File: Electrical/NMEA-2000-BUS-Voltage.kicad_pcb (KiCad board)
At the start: 2 copper layers, 52.1 x 40.6 mm, 12 parts, among them J1 Conn_01x06, SW1 SW_Push, U1 WeMos_D1_mini, U2 LM7805_TO220

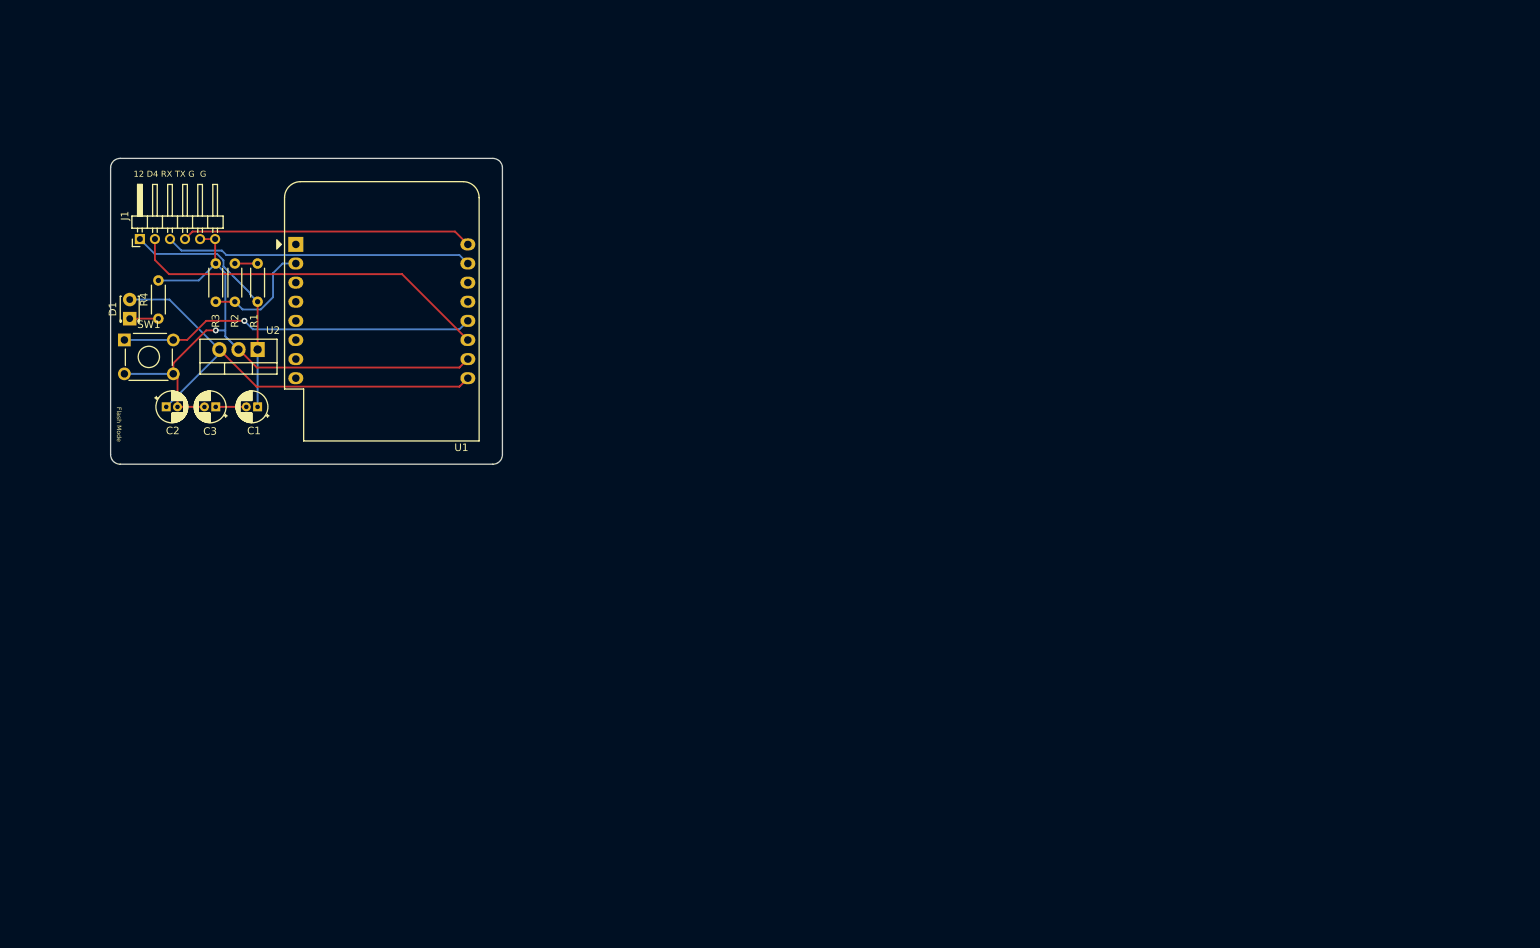
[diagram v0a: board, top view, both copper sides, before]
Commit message: Updated PCB
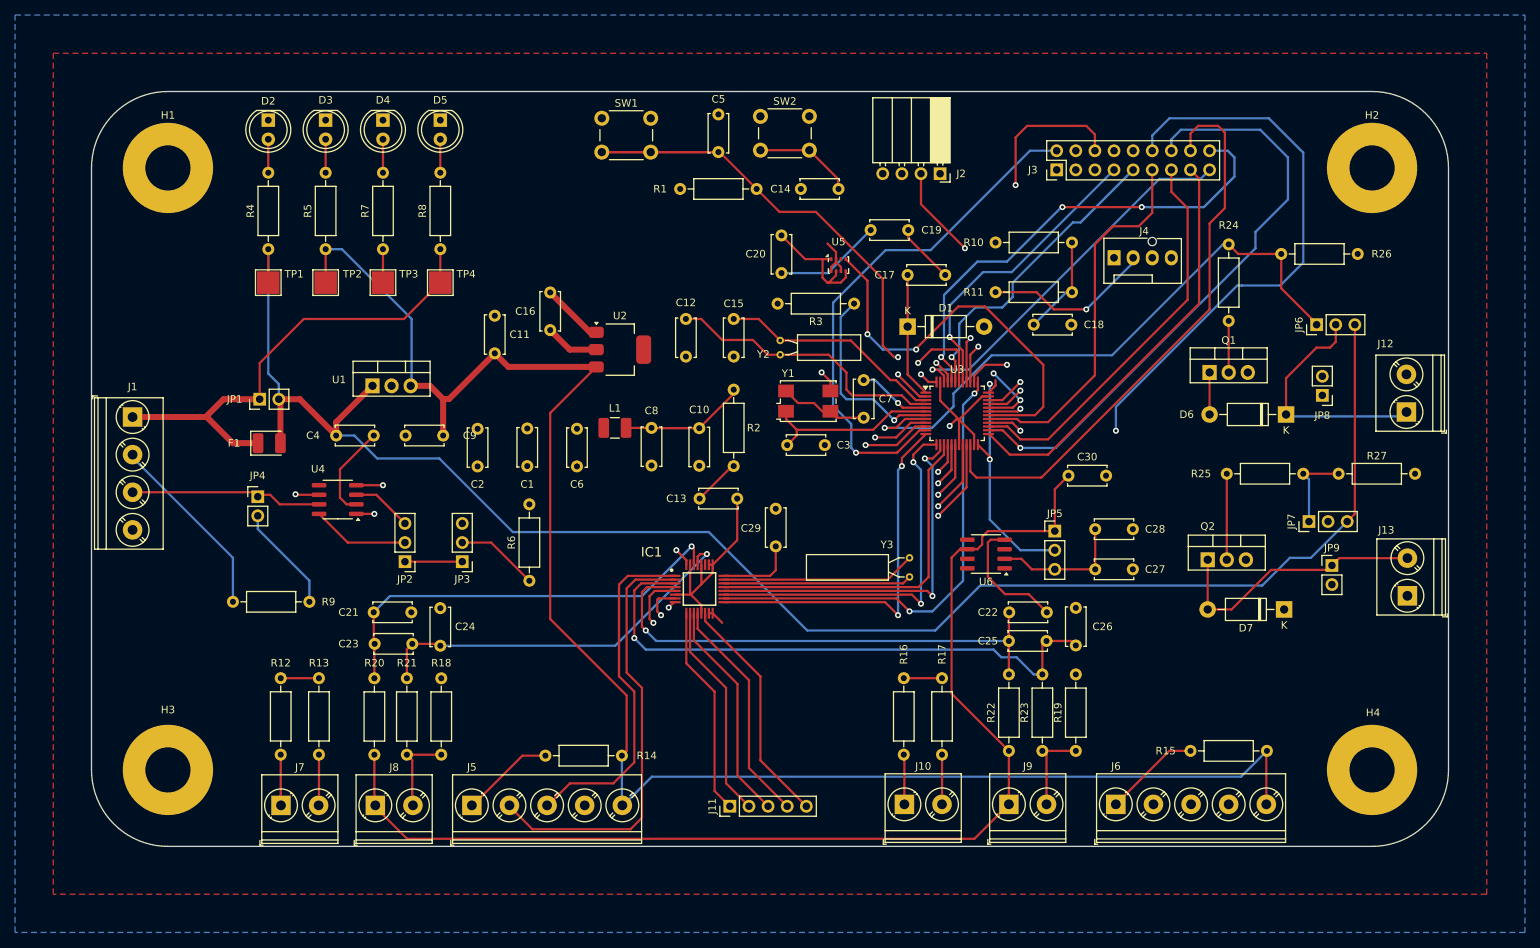
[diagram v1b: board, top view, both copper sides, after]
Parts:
- added C10: 1uF, Capacitor_THT:C_Disc_D5.0mm_W2.5mm_P5.00mm, F.Cu at (139.2, 85.4)
- added C11: 0.33uF, Capacitor_THT:C_Disc_D5.0mm_W2.5mm_P5.00mm, F.Cu at (112.0, 75.4)
- added C12: 20pF, Capacitor_THT:C_Disc_D5.0mm_W2.5mm_P5.00mm, F.Cu at (137.4, 70.9)
- added C13: 0.1uF, Capacitor_THT:C_Disc_D5.0mm_W2.5mm_P5.00mm, F.Cu at (139.2, 94.7)
- added C14: 0.1uF, Capacitor_THT:C_Disc_D5.0mm_W2.5mm_P5.00mm, F.Cu at (152.7, 53.6)
- added C15: 20pF, Capacitor_THT:C_Disc_D5.0mm_W2.5mm_P5.00mm, F.Cu at (143.8, 70.9)
- added C16: 0.1uF, Capacitor_THT:C_Disc_D5.0mm_W2.5mm_P5.00mm, F.Cu at (119.4, 72.3)
- added C17: 0.1uF, Capacitor_THT:C_Disc_D5.0mm_W2.5mm_P5.00mm, F.Cu at (166.9, 65.0)
- added C18: 0.1nF, Capacitor_THT:C_Disc_D5.0mm_W2.5mm_P5.00mm, F.Cu at (183.6, 71.6)
- added C19: 0.1uF, Capacitor_THT:C_Disc_D5.0mm_W2.5mm_P5.00mm, F.Cu at (162.0, 59.1)
- added C20: 0.1uF, Capacitor_THT:C_Disc_D5.0mm_W2.5mm_P5.00mm, F.Cu at (150.1, 64.8)
- added C21: 10nF, Capacitor_THT:C_Disc_D5.0mm_W2.5mm_P5.00mm, F.Cu at (95.9, 109.9)
- added C22: 10nF, Capacitor_THT:C_Disc_D5.0mm_W2.5mm_P5.00mm, F.Cu at (180.4, 109.9)
- added C23: 0.1uF, Capacitor_THT:C_Disc_D5.0mm_W2.5mm_P5.00mm, F.Cu at (96.1, 114.0)
- added C24: 10nF, Capacitor_THT:C_Disc_D5.0mm_W2.5mm_P5.00mm, F.Cu at (104.8, 114.3)
- added C25: 0.1uF, Capacitor_THT:C_Disc_D5.0mm_W2.5mm_P5.00mm, F.Cu at (180.3, 113.7)
- added C26: 10nF, Capacitor_THT:C_Disc_D5.0mm_W2.5mm_P5.00mm, F.Cu at (189.2, 114.3)
- added C27: 1uF, Capacitor_THT:C_Disc_D5.0mm_W2.5mm_P5.00mm, F.Cu at (191.8, 104.1)
- added C28: 0.1uF, Capacitor_THT:C_Disc_D5.0mm_W2.5mm_P5.00mm, F.Cu at (191.8, 98.8)
- added C29: 220nF, Capacitor_THT:C_Disc_D5.0mm_W2.5mm_P5.00mm, F.Cu at (149.4, 101.1)
- added C30: 0.1uF, Capacitor_THT:C_Disc_D5.0mm_W2.5mm_P5.00mm, F.Cu at (188.3, 91.7)
- added C4: 0.33uF, Capacitor_THT:C_Disc_D5.0mm_W2.5mm_P5.00mm, F.Cu at (90.9, 86.4)
- added C5: 0.1uF, Capacitor_THT:C_Disc_D5.0mm_W2.5mm_P5.00mm, F.Cu at (141.7, 43.7)
- added C6: 0.1uF, Capacitor_THT:C_Disc_D5.0mm_W2.5mm_P5.00mm, F.Cu at (122.9, 85.5)
- added C7: 20pF, Capacitor_THT:C_Disc_D5.0mm_W2.5mm_P5.00mm, F.Cu at (161.0, 79.0)
- added C8: 10nF, Capacitor_THT:C_Disc_D5.0mm_W2.5mm_P5.00mm, F.Cu at (132.8, 85.3)
- added C9: 0.1uF, Capacitor_THT:C_Disc_D5.0mm_W2.5mm_P5.00mm, F.Cu at (105.2, 86.4)
- added D2: LED, LED_THT:LED_D5.0mm, F.Cu at (81.9, 44.5)
- added D3: LED, LED_THT:LED_D5.0mm, F.Cu at (89.5, 44.4)
- added D4: LED, LED_THT:LED_D5.0mm, F.Cu at (97.2, 44.5)
- added D5: LED, LED_THT:LED_D5.0mm, F.Cu at (104.8, 44.5)
- added D6: 1N5819, Diode_THT:D_DO-41_SOD81_P10.16mm_Horizontal, F.Cu at (217.2, 83.6)
- added D7: 1N5819, Diode_THT:D_DO-41_SOD81_P10.16mm_Horizontal, F.Cu at (216.9, 109.5)
- added F1: Polyfuse, Diode_SMD:D_1210_3225Metric_Pad1.42x2.65mm_HandSolder, F.Cu at (82.0, 87.4)
- added H1: MountingHole_Pad, MountingHole:MountingHole_6mm_Pad, F.Cu at (68.6, 50.8)
- added H2: MountingHole_Pad, MountingHole:MountingHole_6mm_Pad, F.Cu at (228.6, 50.8)
- added H3: MountingHole_Pad, MountingHole:MountingHole_6mm_Pad, F.Cu at (68.6, 130.8)
- added H4: MountingHole_Pad, MountingHole:MountingHole_6mm_Pad, F.Cu at (228.6, 130.8)
- added IC1: ADS131M08, ADS131M08QPBSRQ1:QFP50P700X700X120-32N, F.Cu at (139.2, 106.8)
- added J10: Conn_01x02, TerminalBlock_Phoenix:TerminalBlock_Phoenix_PT-1,5-2-5.0-H_1x02_P5.00mm_Horizontal, F.Cu at (166.4, 135.4)
- added J11: Conn_01x05, Connector_PinHeader_2.54mm:PinHeader_1x05_P2.54mm_Vertical, F.Cu at (143.3, 135.6)
- added J12: Conn_01x02, TerminalBlock_Phoenix:TerminalBlock_Phoenix_PT-1,5-2-5.0-H_1x02_P5.00mm_Horizontal, F.Cu at (233.2, 83.2)
- added J13: Conn_01x02, TerminalBlock_Phoenix:TerminalBlock_Phoenix_PT-1,5-2-5.0-H_1x02_P5.00mm_Horizontal, F.Cu at (233.3, 107.7)
- added J2: Conn_01x04, Connector_PinSocket_2.54mm:PinSocket_1x04_P2.54mm_Horizontal, F.Cu at (171.2, 51.6)
- added J3: Conn_02x08_Counter_Clockwise, Connector_PinHeader_2.54mm:PinHeader_2x09_P2.54mm_Vertical, F.Cu at (186.7, 51.1)
- added J4: Conn_01x04, Connector:FanPinHeader_1x04_P2.54mm_Vertical, F.Cu at (194.3, 62.7)
- added J5: Conn_01x05, TerminalBlock_Phoenix:TerminalBlock_Phoenix_PT-1,5-5-5.0-H_1x05_P5.00mm_Horizontal, F.Cu at (109.0, 135.5)
- added J6: Conn_01x05, TerminalBlock_Phoenix:TerminalBlock_Phoenix_PT-1,5-5-5.0-H_1x05_P5.00mm_Horizontal, F.Cu at (194.6, 135.4)
- added J7: Conn_01x02, TerminalBlock_Phoenix:TerminalBlock_Phoenix_PT-1,5-2-5.0-H_1x02_P5.00mm_Horizontal, F.Cu at (83.6, 135.5)
- added J8: Conn_01x02, TerminalBlock_Phoenix:TerminalBlock_Phoenix_PT-1,5-2-5.0-H_1x02_P5.00mm_Horizontal, F.Cu at (96.1, 135.5)
- added J9: Conn_01x02, TerminalBlock_Phoenix:TerminalBlock_Phoenix_PT-1,5-2-5.0-H_1x02_P5.00mm_Horizontal, F.Cu at (180.3, 135.4)
- added JP1: Jumper_2_Open, Connector_PinHeader_2.54mm:PinHeader_1x02_P2.54mm_Vertical, F.Cu at (80.8, 81.5)
- added JP2: Jumper_3_Bridged12, Connector_PinHeader_2.54mm:PinHeader_1x03_P2.54mm_Vertical, F.Cu at (100.1, 103.1)
- added JP3: Jumper_3_Bridged12, Connector_PinHeader_2.54mm:PinHeader_1x03_P2.54mm_Vertical, F.Cu at (107.7, 103.1)
- added JP4: Jumper_2_Open, Connector_PinHeader_2.54mm:PinHeader_1x02_P2.54mm_Vertical, F.Cu at (80.5, 94.5)
- added JP5: Jumper_3_Bridged12, Connector_PinHeader_2.54mm:PinHeader_1x03_P2.54mm_Vertical, F.Cu at (186.4, 99.1)
- added JP6: Jumper_3_Bridged12, Connector_PinHeader_2.54mm:PinHeader_1x03_P2.54mm_Vertical, F.Cu at (221.2, 71.6)
- added JP7: Jumper_3_Bridged12, Connector_PinHeader_2.54mm:PinHeader_1x03_P2.54mm_Vertical, F.Cu at (220.2, 97.8)
- added JP8: Jumper_2_Bridged, Connector_PinHeader_2.54mm:PinHeader_1x02_P2.54mm_Vertical, F.Cu at (222.0, 81.0)
- added JP9: Jumper_2_Bridged, Connector_PinHeader_2.54mm:PinHeader_1x02_P2.54mm_Vertical, F.Cu at (223.3, 103.6)
- added L1: CBG322513U102T, Inductor_SMD:L_1210_3225Metric_Pad1.42x2.65mm_HandSolder, F.Cu at (128.0, 85.3)
- added Q1: IRFZ44N, Package_TO_SOT_THT:TO-220-3_Vertical, F.Cu at (207.0, 78.0)
- added Q2: IRFZ44N, Package_TO_SOT_THT:TO-220-3_Vertical, F.Cu at (206.8, 102.9)
- added R10: 10k, Resistor_THT:R_Axial_DIN0207_L6.3mm_D2.5mm_P10.16mm_Horizontal, F.Cu at (178.6, 60.7)
- added R11: 3.3k, Resistor_THT:R_Axial_DIN0207_L6.3mm_D2.5mm_P10.16mm_Horizontal, F.Cu at (188.7, 67.3)
- added R12: 10k, Resistor_THT:R_Axial_DIN0207_L6.3mm_D2.5mm_P10.16mm_Horizontal, F.Cu at (83.6, 128.8)
- added R13: 4k7, Resistor_THT:R_Axial_DIN0207_L6.3mm_D2.5mm_P10.16mm_Horizontal, F.Cu at (88.6, 118.6)
- added R14: 10k, Resistor_THT:R_Axial_DIN0207_L6.3mm_D2.5mm_P10.16mm_Horizontal, F.Cu at (128.9, 128.9)
- added R15: 10k, Resistor_THT:R_Axial_DIN0207_L6.3mm_D2.5mm_P10.16mm_Horizontal, F.Cu at (204.5, 128.3)
- added R16: 10k, Resistor_THT:R_Axial_DIN0207_L6.3mm_D2.5mm_P10.16mm_Horizontal, F.Cu at (166.4, 128.8)
- added R17: 4k7, Resistor_THT:R_Axial_DIN0207_L6.3mm_D2.5mm_P10.16mm_Horizontal, F.Cu at (171.4, 118.6)
- added R18: 10k, Resistor_THT:R_Axial_DIN0207_L6.3mm_D2.5mm_P10.16mm_Horizontal, F.Cu at (104.9, 128.8)
- added R19: 10k, Resistor_THT:R_Axial_DIN0207_L6.3mm_D2.5mm_P10.16mm_Horizontal, F.Cu at (189.2, 128.3)
- added R20: 1k, Resistor_THT:R_Axial_DIN0207_L6.3mm_D2.5mm_P10.16mm_Horizontal, F.Cu at (96.0, 128.8)
- added R21: 1k, Resistor_THT:R_Axial_DIN0207_L6.3mm_D2.5mm_P10.16mm_Horizontal, F.Cu at (100.3, 128.8)
- added R22: 1k, Resistor_THT:R_Axial_DIN0207_L6.3mm_D2.5mm_P10.16mm_Horizontal, F.Cu at (180.3, 128.3)
- added R23: 1k, Resistor_THT:R_Axial_DIN0207_L6.3mm_D2.5mm_P10.16mm_Horizontal, F.Cu at (184.8, 128.3)
- added R24: 120R, Resistor_THT:R_Axial_DIN0207_L6.3mm_D2.5mm_P10.16mm_Horizontal, F.Cu at (209.6, 61.0)
- added R25: 120R, Resistor_THT:R_Axial_DIN0207_L6.3mm_D2.5mm_P10.16mm_Horizontal, F.Cu at (219.5, 91.4)
- added R26: 10k, Resistor_THT:R_Axial_DIN0207_L6.3mm_D2.5mm_P10.16mm_Horizontal, F.Cu at (216.5, 62.2)
- added R27: 10k, Resistor_THT:R_Axial_DIN0207_L6.3mm_D2.5mm_P10.16mm_Horizontal, F.Cu at (224.2, 91.4)
- added R5: 470R, Resistor_THT:R_Axial_DIN0207_L6.3mm_D2.5mm_P10.16mm_Horizontal, F.Cu at (89.5, 61.6)
- added R6: 10k, Resistor_THT:R_Axial_DIN0207_L6.3mm_D2.5mm_P10.16mm_Horizontal, F.Cu at (116.6, 105.7)
- added R7: 330R, Resistor_THT:R_Axial_DIN0207_L6.3mm_D2.5mm_P10.16mm_Horizontal, F.Cu at (97.2, 61.6)
- added R8: 1k5, Resistor_THT:R_Axial_DIN0207_L6.3mm_D2.5mm_P10.16mm_Horizontal, F.Cu at (104.8, 61.6)
- added R9: 120R, Resistor_THT:R_Axial_DIN0207_L6.3mm_D2.5mm_P10.16mm_Horizontal, F.Cu at (87.4, 108.5)
- added SW2: SW_Push, Button_Switch_THT:SW_PUSH_6mm, F.Cu at (147.3, 43.9)
- added TP1: 12V, TestPoint:TestPoint_Pad_3.0x3.0mm, F.Cu at (81.9, 66.0)
- added TP2: 5V, TestPoint:TestPoint_Pad_3.0x3.0mm, F.Cu at (89.5, 66.0)
- added TP3: 3.3V, TestPoint:TestPoint_Pad_3.0x3.0mm, F.Cu at (97.2, 66.0)
- added TP4: VMot, TestPoint:TestPoint_Pad_3.0x3.0mm, F.Cu at (104.8, 66.0)
- added U3: STM32G431CBTx, Package_QFP:LQFP-48_7x7mm_P0.5mm, F.Cu at (173.5, 83.4)
- added U4: SN65HVD230, Package_SO:SOIC-8_3.9x4.9mm_P1.27mm, F.Cu at (91.1, 94.9)
- added U5: BMP280, N2K-influx:Bosch_LGA-8_2x2.5mm_P0.65mm_ClockwisePinNumbering, F.Cu at (157.7, 63.7)
- added U6: ADR4533, Package_SO:SOIC-8_3.9x4.9mm_P1.27mm, F.Cu at (177.3, 102.1)
- added Y1: K7A080002020, Crystal:Crystal_SMD_7050-4Pin_7.0x5.0mm, F.Cu at (153.7, 81.8)
- added Y2: X308032768KGB2SC, Crystal:Crystal_C38-LF_D3.0mm_L8.0mm_Horizontal, F.Cu at (149.9, 75.6)
- added Y3: 20kHz Crystal, Crystal:Crystal_AT310_D3.0mm_L10.0mm_Horizontal, F.Cu at (167.1, 102.6)
- C1: value 0.2uF -> 0.1uF; footprint Capacitor_THT:CP_Radial_D4.0mm_P1.50mm -> Capacitor_THT:C_Disc_D5.0mm_W2.5mm_P5.00mm
- C2: footprint Capacitor_THT:CP_Radial_D4.0mm_P1.50mm -> Capacitor_THT:C_Disc_D5.0mm_W2.5mm_P5.00mm
- C3: value 0.1uF -> 20pF; footprint Capacitor_THT:CP_Radial_D4.0mm_P1.50mm -> Capacitor_THT:C_Disc_D5.0mm_W2.5mm_P5.00mm
- D1: value LED -> 1N5819; footprint LED_THT:LED_D1.8mm_W3.3mm_H2.4mm -> Diode_THT:D_DO-41_SOD81_P10.16mm_Horizontal
- J1: value Conn_01x06 -> Conn_01x04; footprint Connector_PinHeader_2.00mm:PinHeader_1x06_P2.00mm_Horizontal -> TerminalBlock_Phoenix:TerminalBlock_Phoenix_PT-1,5-4-5.0-H_1x04_P5.00mm_Horizontal
- R1: footprint Resistor_THT:R_Axial_DIN0204_L3.6mm_D1.6mm_P5.08mm_Horizontal -> Resistor_THT:R_Axial_DIN0207_L6.3mm_D2.5mm_P10.16mm_Horizontal
- R2: value 20k -> 0R; footprint Resistor_THT:R_Axial_DIN0204_L3.6mm_D1.6mm_P5.08mm_Horizontal -> Resistor_THT:R_Axial_DIN0207_L6.3mm_D2.5mm_P10.16mm_Horizontal
- R3: value 120k -> 10k; footprint Resistor_THT:R_Axial_DIN0204_L3.6mm_D1.6mm_P5.08mm_Horizontal -> Resistor_THT:R_Axial_DIN0207_L6.3mm_D2.5mm_P10.16mm_Horizontal
- R4: value 1k -> 1.2k; footprint Resistor_THT:R_Axial_DIN0204_L3.6mm_D1.6mm_P5.08mm_Horizontal -> Resistor_THT:R_Axial_DIN0207_L6.3mm_D2.5mm_P10.16mm_Horizontal
- SW1: footprint Button_Switch_THT:SW_TH_Tactile_Omron_B3F-10xx -> Button_Switch_THT:SW_PUSH_6mm
- U1: value WeMos_D1_mini -> LM7805_TO220; footprint Module:WEMOS_D1_mini_light -> Package_TO_SOT_THT:TO-220-3_Vertical
- U2: value LM7805_TO220 -> AMS1117-3.3; footprint Package_TO_SOT_THT:TO-220-3_Vertical -> Package_TO_SOT_SMD:SOT-223-3_TabPin2
- moved D1 103.4 mm to (166.9, 71.9), turned to 0 degrees
- moved R3 84.8 mm to (159.8, 68.8), turned to 180 degrees
- moved C3 76.1 mm to (150.9, 87.6), turned to 0 degrees
- moved SW1 70.0 mm to (126.2, 44.2)
- moved R2 68.4 mm to (143.8, 80.3)
- moved R1 58.1 mm to (136.7, 53.6), turned to 0 degrees
- moved U2 48.2 mm to (128.7, 74.9), turned to 0 degrees
- moved C2 41.5 mm to (109.7, 85.5), turned to -90 degrees
- moved C1 36.0 mm to (116.3, 85.4), turned to -90 degrees
- moved J1 23.7 mm to (63.9, 83.9), turned to -90 degrees
- moved U1 21.4 mm to (95.8, 79.8)
- moved R4 17.3 mm to (81.9, 61.6)
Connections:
- C1 pad 1: +12V -> +3.3V
- C1 pad 2: Net-(C1-Pad2) -> GND
- C2 pad 1: +5V -> +3.3V
- C3 pad 1: Net-(C1-Pad2) -> Net-(U3-PF1)
- D1 pad 2: +5V -> +3.3V
- J1 pad 1: +12V -> VMot
- J1 pad 2: /D4 -> /CAN_L
- J1 pad 3: /RX -> /CAN_H
- J1 pad 4: /TX -> GND
- R1 pad 1: +12V -> GND
- R1 pad 2: /A0 -> Net-(U3-PB8)
- R2 pad 1: /A0 -> +3.3VA
- R2 pad 2: Net-(R2-Pad2) -> /V_{ref}+
- R3 pad 1: Net-(R2-Pad2) -> /EN
- R3 pad 2: GND -> +3.3V
- R4 pad 1: Net-(D1-K) -> +12V
- R4 pad 2: GND -> Net-(D2-A)
- SW1 pad 1: /FLASH -> +3.3V
- SW1 pad 2: GND -> Net-(U3-PB8)
- U1 pad 1: unconnected-(U1-~{RST}-Pad1) -> +12V
- U1 pad 2: /A0 -> GND
- U1 pad 3: unconnected-(U1-D0-Pad3) -> +5V
- U2 pad 1: +12V -> GND
- U2 pad 2: GND -> +3.3V
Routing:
- net +5V: track 60.7 -> 292.3 mm
- net +12V: track 33.6 -> 259.5 mm
- net /Sensor/V_{ref}: track 0.00 -> 154.8 mm
- net /CAN_{RX}: track 0.00 -> 122.6 mm, vias 0 -> 2
- net /CAN_{TX}: track 0.00 -> 114.9 mm, vias 0 -> 2
- net /PB14: track 0.00 -> 92.9 mm, vias 0 -> 2
- net /TX: track 38.7 -> 128.0 mm, vias 0 -> 1
- net /Sensor/AIN5P: track 0.00 -> 88.2 mm, vias 0 -> 1
- net +3.3V: track 0.00 -> 87.3 mm, vias 0 -> 3
- net /EN: track 0.00 -> 85.0 mm, vias 0 -> 1
- net REL2: track 0.00 -> 83.4 mm, vias 0 -> 1
- net REL1: track 0.00 -> 81.7 mm, vias 0 -> 1
- net /PB12: track 0.00 -> 80.4 mm, vias 0 -> 1
- net Net-(U3-PB8): track 0.00 -> 79.9 mm, vias 0 -> 2
- net /Sensor/AIN5N: track 0.00 -> 79.0 mm, vias 0 -> 1
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- added copper zone on F.Cu, net +3.3V
- added copper zone on B.Cu, net GND
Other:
- board size 52.1 x 40.6 mm -> 180.3 x 100.3 mm
- copper layers 2 -> 4
- board text removed: "12 D4 RX TX G G"
- board text removed: "Flash Mode"
